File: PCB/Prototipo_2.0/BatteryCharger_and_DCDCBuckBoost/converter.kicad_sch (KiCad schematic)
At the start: 1 part

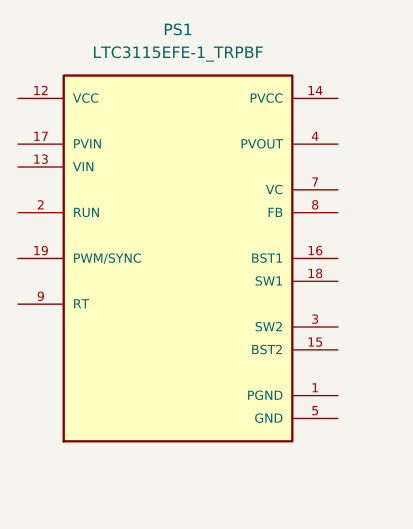
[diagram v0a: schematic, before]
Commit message: .
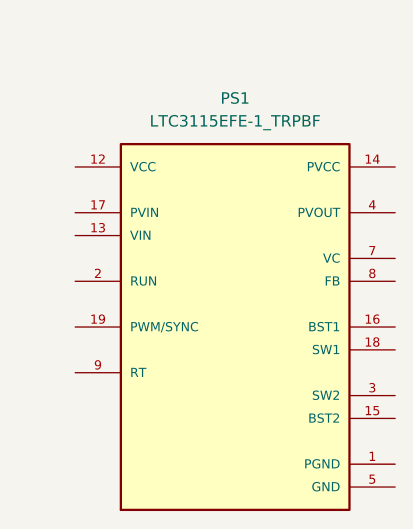
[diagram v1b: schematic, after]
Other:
- company: (none) -> UPM-Nizar El Azeouzi Amine
- title: (none) -> Converter_DCDC_BuckBoost
- moved on the sheet: PS1
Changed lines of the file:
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@@
 	(generator_version "9.0")
 	(paper "A4")
+	(title_block
+		(title "Converter_DCDC_BuckBoost")
+		(date "2026-06-05")
+		(company "UPM-Nizar El Azeouzi Amine")
+	)
 	(symbol
 		(lib_id "LTC3115EFE-1_TRPBF:LTC3115EFE-1_TRPBF")
-		(at 135.89 71.12 0)
+		(at 142.24 78.74 0)
 		(unit 1)
 		(exclude_from_sim no)
@@
 		(fields_autoplaced yes)
 		(property "Reference" "PS1"
-			(at 135.89 45.72 0)
+			(at 142.24 53.34 0)
 			(effects
 				(font
@@
 		)
 		(property "Value" "LTC3115EFE-1_TRPBF"
-			(at 135.89 48.26 0)
+			(at 142.24 55.88 0)
 			(effects
 				(font
@@
 		)
 		(property "Footprint" "LTC3115EFE-1_TRPBF:CONV_LTC3115EFE-1_TRPBF"
-			(at 135.89 71.12 0)
+			(at 142.24 78.74 0)
 			(effects
 				(font
@@
 		)
 		(property "Datasheet" ""
-			(at 135.89 71.12 0)
+			(at 142.24 78.74 0)
 			(effects
 				(font
@@
 		)
 		(property "Description" ""
-			(at 135.89 71.12 0)
+			(at 142.24 78.74 0)
 			(effects
 				(font
@@
 		)
 		(property "MF" "Analog Devices"
-			(at 135.89 71.12 0)
+			(at 142.24 78.74 0)
 			(effects
 				(font
@@
 		)
 		(property "MAXIMUM_PACKAGE_HEIGHT" "1.2mm"
-			(at 135.89 71.12 0)
+			(at 142.24 78.74 0)
 			(effects
 				(font
@@
 		)
 		(property "Package" "TSSOP -20 Analog Devices"
-			(at 135.89 71.12 0)
+			(at 142.24 78.74 0)
 			(effects
 				(font
@@
 		)
 		(property "Price" "None"
-			(at 135.89 71.12 0)
+			(at 142.24 78.74 0)
 			(effects
 				(font
@@
 		)
 		(property "Check_prices" "https://www.snapeda.com/parts/LTC3115EFE-1%23TRPBF/Analog+Devices/view-part/?ref=eda"
-			(at 135.89 71.12 0)
+			(at 142.24 78.74 0)
 			(effects
 				(font
@@
 		)
 		(property "STANDARD" "Manufacturer Recommendations"
-			(at 135.89 71.12 0)
+			(at 142.24 78.74 0)
 			(effects
 				(font
@@
 		)
 		(property "PARTREV" "E"
-			(at 135.89 71.12 0)
+			(at 142.24 78.74 0)
 			(effects
 				(font
@@
 		)
 		(property "SnapEDA_Link" "https://www.snapeda.com/parts/LTC3115EFE-1%23TRPBF/Analog+Devices/view-part/?ref=snap"
-			(at 135.89 71.12 0)
+			(at 142.24 78.74 0)
 			(effects
 				(font
@@
 		)
 		(property "MP" "LTC3115EFE-1#TRPBF"
-			(at 135.89 71.12 0)
+			(at 142.24 78.74 0)
 			(effects
 				(font
@@
 		)
 		(property "Purchase-URL" "https://www.snapeda.com/api/url_track_click_mouser/?unipart_id=4338510&manufacturer=Analog Devices&part_name=LTC3115EFE-1#TRPBF&search_term=ltc3115efe-1#trpbf"
-			(at 135.89 71.12 0)
+			(at 142.24 78.74 0)
 			(effects
 				(font
@@
 		)
 		(property "Description_1" "40V, 2A Synchronous Buck-Boost DC/DC Converter"
-			(at 135.89 71.12 0)
+			(at 142.24 78.74 0)
 			(effects
 				(font
@@
 		)
 		(property "Availability" "In Stock"
-			(at 135.89 71.12 0)
+			(at 142.24 78.74 0)
 			(effects
 				(font
@@
 		)
 		(property "MANUFACTURER" "Analog Devices"
-			(at 135.89 71.12 0)
+			(at 142.24 78.74 0)
 			(effects
 				(font
